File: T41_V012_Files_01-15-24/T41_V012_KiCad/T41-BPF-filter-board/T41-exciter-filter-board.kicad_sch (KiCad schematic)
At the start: 262 parts, among them J1 TO PA, J2 FROM EXCITE, J3 12-13.8V, J4 Bands, J5 TO RECEIVE, J6 FROM LPF, U1 MASWSS0179, U10 MASWSS0179, U11 SN74LVC1G04DCK, U12 MASWSS0179, U13 MASWSS0179, U14 SN74LVC1G04DCK, U15 MASWSS0179, U16 MASWSS0179, U17 SN74LVC1G04DCK, U18 MASWSS0179, U19 MASWSS0179, U2 SN74LVC1G04DCK, U20 SN74LVC1G04DCK, U21 MASWSS0179, U22 LM1117T-3.3, U23 SN74LVC1G04DCK, U24 MASWSS0179, U25 MASWSS0179, U26 SN74LVC1G04DCK, U27 MASWSS0179, U28 MASWSS0179, U29 SN74LVC1G04DCK, U3 MASWSS0179, U30 MASWSS0179, U31 MASWSS0179, U35 MCP23017_SO, U36 MASWSS0179, U37 SN74LVC1G04DCK, U4 MASWSS0179, U5 SN74LVC1G04DCK, U6 MASWSS0179, U7 MASWSS0179, U8 SN74LVC1G04DCK, U9 MASWSS0179

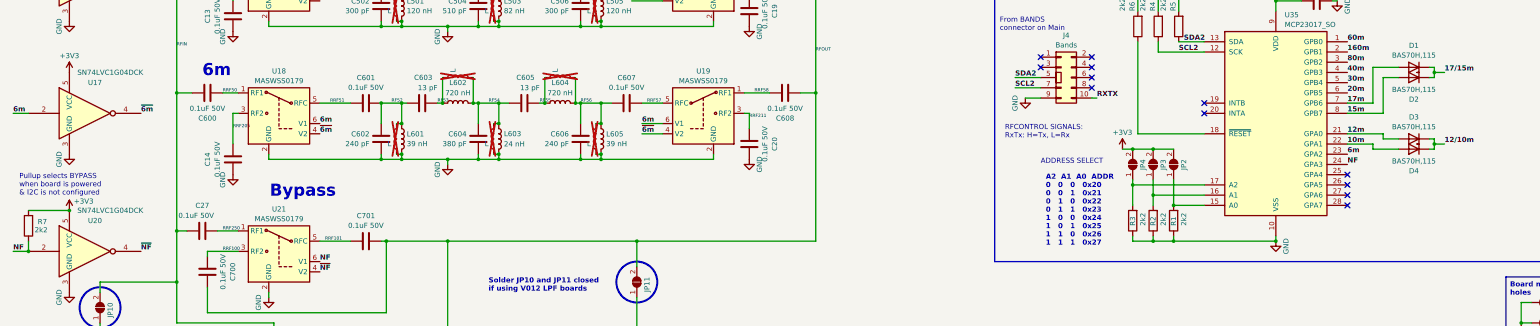
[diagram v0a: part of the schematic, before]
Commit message: Added pulldown resistors to 12/10 and 17/15 diode combiners
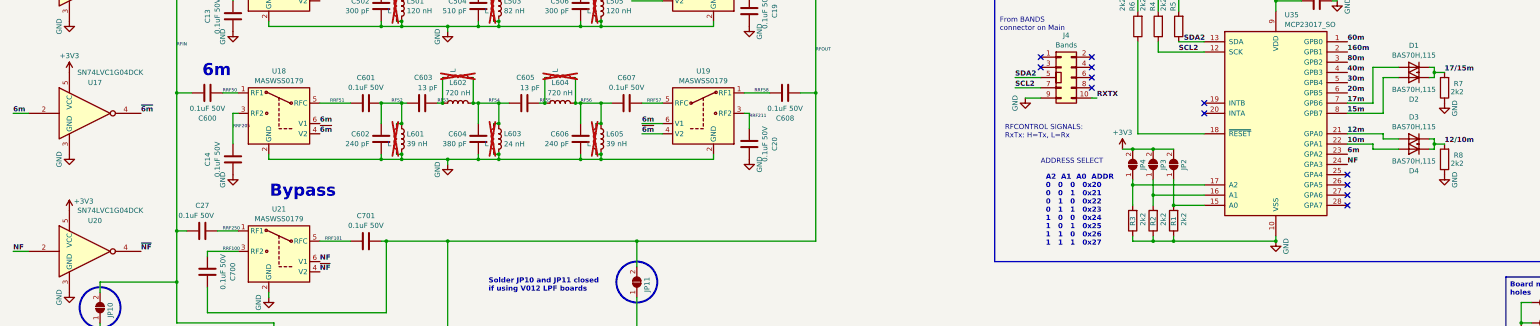
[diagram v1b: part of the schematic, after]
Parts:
- added R8: 2k2, Resistor_SMD:R_1206_3216Metric, symbol Device:R
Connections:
- net +3V3: no longer R7.2
- net 12/10m: now also R8.2
- net 17/15m: now also R7.2
- net GND: now also R7.1, R8.1
- net NF: no longer R7.1
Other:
- note removed: "Pullup selects BYPASS when board is powered & I2C is not configured"
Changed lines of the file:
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@@
 	)
 	(junction
-		(at 16.51 227.33)
-		(diameter 0)
-		(color 0 0 0 0)
-	)
-	(junction
 		(at 109.22 74.93)
 		(diameter 0)
@@
 	)
 	(junction
-		(at 26.67 217.17)
-		(diameter 0)
-		(color 0 0 0 0)
-	)
-	(junction
 		(at 133.35 35.56)
 		(diameter 0)
@@
 	(wire
 		(pts
-			(xy 16.51 217.17) (xy 26.67 217.17)
-		)
-		(stroke
-			(width 0)
-			(type default)
-		)
-	)
-	(wire
-		(pts
 			(xy 307.34 43.18) (xy 308.61 43.18)
 		)
@@
 	(wire
 		(pts
-			(xy 16.51 224.79) (xy 16.51 227.33)
-		)
-		(stroke
-			(width 0)
-			(type default)
-		)
-	)
-	(wire
-		(pts
 			(xy 120.65 204.47) (xy 120.65 205.74)
 		)
@@
 		)
 	)
-	(text "Pullup selects BYPASS\nwhen board is powered\n& I2C is not configured"
-		(exclude_from_sim no)
-		(at 14.224 210.82 0)
-		(effects
-			(font
-				(size 1.27 1.27)
-			)
-			(justify left)
-		)
-	)
 	(text "RFCONTROL SIGNALS:\nRxTx: H=Tx, L=Rx"
 		(exclude_from_sim no)
@@
 	)
 	(symbol
-		(lib_id "Device:C")
-		(at 100.33 30.48 90)
+		(lib_id "Device:R")
+		(at 368.3 204.47 180)
 		(unit 1)
 		(exclude_from_sim no)
@@
 		(on_board yes)
 		(dnp no)
-		(fields_autoplaced yes)
-		(property "Reference" "C101"
-			(at 100.33 24.1767 90)
+		(property "Reference" "R8"
+			(at 370.586 203.454 0)
 			(effects
 				(font
 					(size 1.27 1.27)
 				)
+				(justify right)
 			)
 		)
-		(property "Value" "0.1uF 50V"
-			(at 100.33 26.6009 90)
+		(property "Value" "2k2"
+			(at 369.824 205.486 0)
 			(effects
 				(font
 					(size 1.27 1.27)
 				)
+				(justify right)
 			)
 		)
-		(property "Footprint" "Capacitor_SMD:C_1206_3216Metric"
-			(at 104.14 29.5148 0)
+		(property "Footprint" "Resistor_SMD:R_1206_3216Metric"
+			(at 370.078 204.47 90)
 			(effects
 				(font
@@
 		)
 		(property "Datasheet" "~"
-			(at 100.33 30.48 0)
+			(at 368.3 204.47 0)
 			(effects
 				(font
@@
 		)
 		(property "Description" ""
-			(at 100.33 30.48 0)
+			(at 368.3 204.47 0)
 			(effects
 				(font
@@
 			)
 		)
-		(property "Mouser Part Number" "C1206C104K5RACTU"
-			(at 100.33 30.48 0)
+		(property "Mouser Part Number" "652-CR1206FX-2201ELF"
+			(at 368.3 204.47 0)
 			(effects
 				(font
@@
 			(project "T41-exciter-filter-board"
 				(path "/56a77fe5-f7a5-414c-a0f7-d659071572ee"
-					(reference "C101")
+					(reference "R8")
 					(unit 1)
 				)
@@
 	)
 	(symbol
-		(lib_id "Device:R")
-		(at 16.51 220.98 180)
+		(lib_id "Device:C")
+		(at 100.33 30.48 90)
 		(unit 1)
 		(exclude_from_sim no)
@@
 		(on_board yes)
 		(dnp no)
-		(property "Reference" "R7"
-			(at 18.796 219.964 0)
+		(fields_autoplaced yes)
+		(property "Reference" "C101"
+			(at 100.33 24.1767 90)
 			(effects
 				(font
 					(size 1.27 1.27)
 				)
-				(justify right)
 			)
 		)
-		(property "Value" "2k2"
-			(at 18.034 221.996 0)
+		(property "Value" "0.1uF 50V"
+			(at 100.33 26.6009 90)
 			(effects
 				(font
 					(size 1.27 1.27)
 				)
-				(justify right)
 			)
 		)
-		(property "Footprint" "Resistor_SMD:R_1206_3216Metric"
-			(at 18.288 220.98 90)
+		(property "Footprint" "Capacitor_SMD:C_1206_3216Metric"
+			(at 104.14 29.5148 0)
 			(effects
 				(font
@@
 		)
 		(property "Datasheet" "~"
-			(at 16.51 220.98 0)
+			(at 100.33 30.48 0)
 			(effects
 				(font
@@
 		)
 		(property "Description" ""
-			(at 16.51 220.98 0)
+			(at 100.33 30.48 0)
 			(effects
 				(font
@@
 			)
 		)
-		(property "Mouser Part Number" "652-CR1206FX-2201ELF"
-			(at 16.51 220.98 0)
+		(property "Mouser Part Number" "C1206C104K5RACTU"
+			(at 100.33 30.48 0)
 			(effects
 				(font
@@
 			(project "T41-exciter-filter-board"
 				(path "/56a77fe5-f7a5-414c-a0f7-d659071572ee"
-					(reference "R7")
+					(reference "C101")
 					(unit 1)
 				)
@@
 	)
 	(symbol
+		(lib_id "power:GND")
+		(at 368.3 208.28 0)
+		(mirror y)
+		(unit 1)
+		(exclude_from_sim no)
+		(in_bom yes)
+		(on_board yes)
+		(dnp no)
+		(property "Reference" "#PWR061"
+			(at 368.3 214.63 0)
+			(effects
+				(font
+					(size 1.27 1.27)
+				)
+				(hide yes)
+			)
+		)
+		(property "Value" "GND"
+			(at 370.84 209.55 90)
+			(effects
+				(font
+					(size 1.27 1.27)
+				)
+			)
+		)
+		(property "Footprint" ""
+			(at 368.3 208.28 0)
+			(effects
+				(font
+					(size 1.27 1.27)
+				)
+				(hide yes)
+			)
+		)
+		(property "Datasheet" ""
+			(at 368.3 208.28 0)
+			(effects
+				(font
+					(size 1.27 1.27)
+				)
+				(hide yes)
+			)
+		)
+		(property "Description" ""
+			(at 368.3 208.28 0)
+			(effects
+				(font
+					(size 1.27 1.27)
+				)
+				(hide yes)
+			)
+		)
+		(pin "1"
+		)
+		(instances
+			(project "T41-exciter-filter-board"
+				(path "/56a77fe5-f7a5-414c-a0f7-d659071572ee"
+					(reference "#PWR061")
+					(unit 1)
+				)
+			)
+		)
+	)
+	(symbol
 		(lib_id "Device:C")
 		(at 139.7 190.5 270)
@@
 	)
 	(symbol
+		(lib_id "Device:R")
+		(at 368.3 186.69 180)
+		(unit 1)
+		(exclude_from_sim no)
+		(in_bom yes)
+		(on_board yes)
+		(dnp no)
+		(property "Reference" "R7"
+			(at 370.586 185.674 0)
+			(effects
+				(font
+					(size 1.27 1.27)
+				)
+				(justify right)
+			)
+		)
+		(property "Value" "2k2"
+			(at 369.824 187.706 0)
+			(effects
+				(font
+					(size 1.27 1.27)
+				)
+				(justify right)
+			)
+		)
+		(property "Footprint" "Resistor_SMD:R_1206_3216Metric"
+			(at 370.078 186.69 90)
+			(effects
+				(font
+					(size 1.27 1.27)
+				)
+				(hide yes)
+			)
+		)
+		(property "Datasheet" "~"
+			(at 368.3 186.69 0)
+			(effects
+				(font
+					(size 1.27 1.27)
+				)
+				(hide yes)
+			)
+		)
+		(property "Description" ""
+			(at 368.3 186.69 0)
+			(effects
+				(font
+					(size 1.27 1.27)
+				)
+				(hide yes)
+			)
+		)
+		(property "Mouser Part Number" "652-CR1206FX-2201ELF"
+			(at 368.3 186.69 0)
+			(effects
+				(font
+					(size 1.27 1.27)
+				)
+				(hide yes)
+			)
+		)
+		(pin "2"
+		)
+		(pin "1"
+		)
+		(instances
+			(project "T41-exciter-filter-board"
+				(path "/56a77fe5-f7a5-414c-a0f7-d659071572ee"
+					(reference "R7")
+					(unit 1)
+				)
+			)
+		)
+	)
+	(symbol
 		(lib_id "power:+3V3")
 		(at 26.67 22.86 0)
@@
 					(unit 1)
 				)
+			)
+		)
+	)
+	(symbol
+		(lib_id "power:GND")
+		(at 368.3 190.5 0)
+		(mirror y)
+		(unit 1)
+		(exclude_from_sim no)
+		(in_bom yes)
+		(on_board yes)
+		(dnp no)
+		(property "Reference" "#PWR041"
+			(at 368.3 196.85 0)
+			(effects
+				(font
+					(size 1.27 1.27)
+				)
+				(hide yes)
+			)
+		)
+		(property "Value" "GND"
+			(at 370.84 191.77 90)
+			(effects
+				(font
+					(size 1.27 1.27)
+				)
+			)
+		)
+		(property "Footprint" ""
+			(at 368.3 190.5 0)
+			(effects
+				(font
+					(size 1.27 1.27)
+				)
+				(hide yes)
+			)
+		)
+		(property "Datasheet" ""
+			(at 368.3 190.5 0)
+			(effects
+				(font
+					(size 1.27 1.27)
+				)
+				(hide yes)
+			)
+		)
+		(property "Description" ""
+			(at 368.3 190.5 0)
+			(effects
+				(font
+					(size 1.27 1.27)
+				)
+				(hide yes)
+			)
+		)
+		(pin "1"
+		)
+		(instances
+			(project "T41-exciter-filter-board"
+				(path "/56a77fe5-f7a5-414c-a0f7-d659071572ee"
+					(reference "#PWR041")
+					(unit 1)
+				)
